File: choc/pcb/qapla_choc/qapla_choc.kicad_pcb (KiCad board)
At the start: 2 copper layers, 154.4 x 126.1 mm, 72 parts

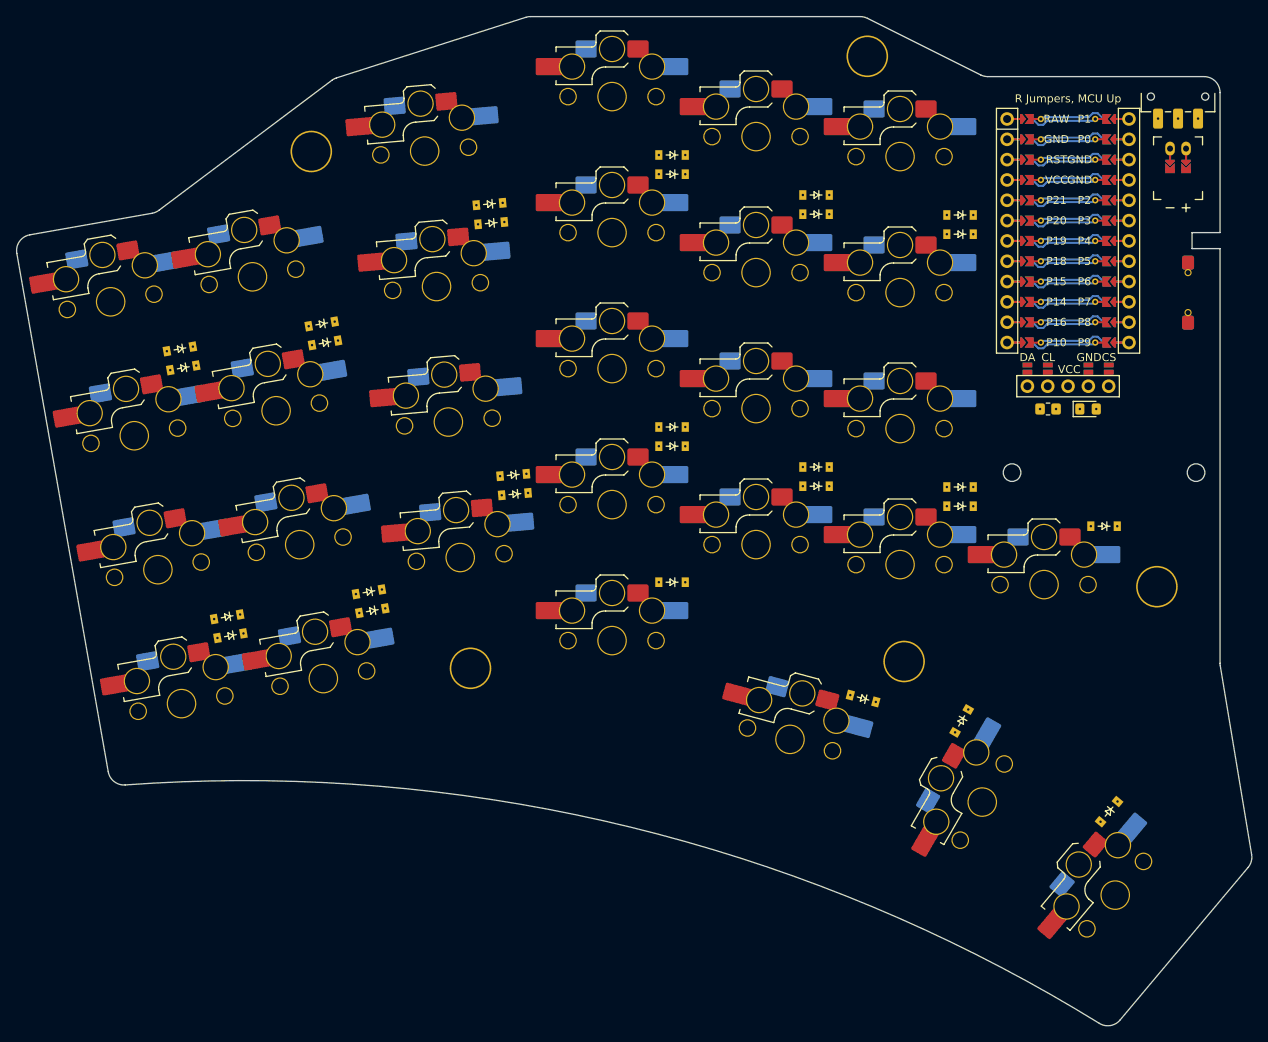
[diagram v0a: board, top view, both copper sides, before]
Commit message: MX Keyboard has a batleth
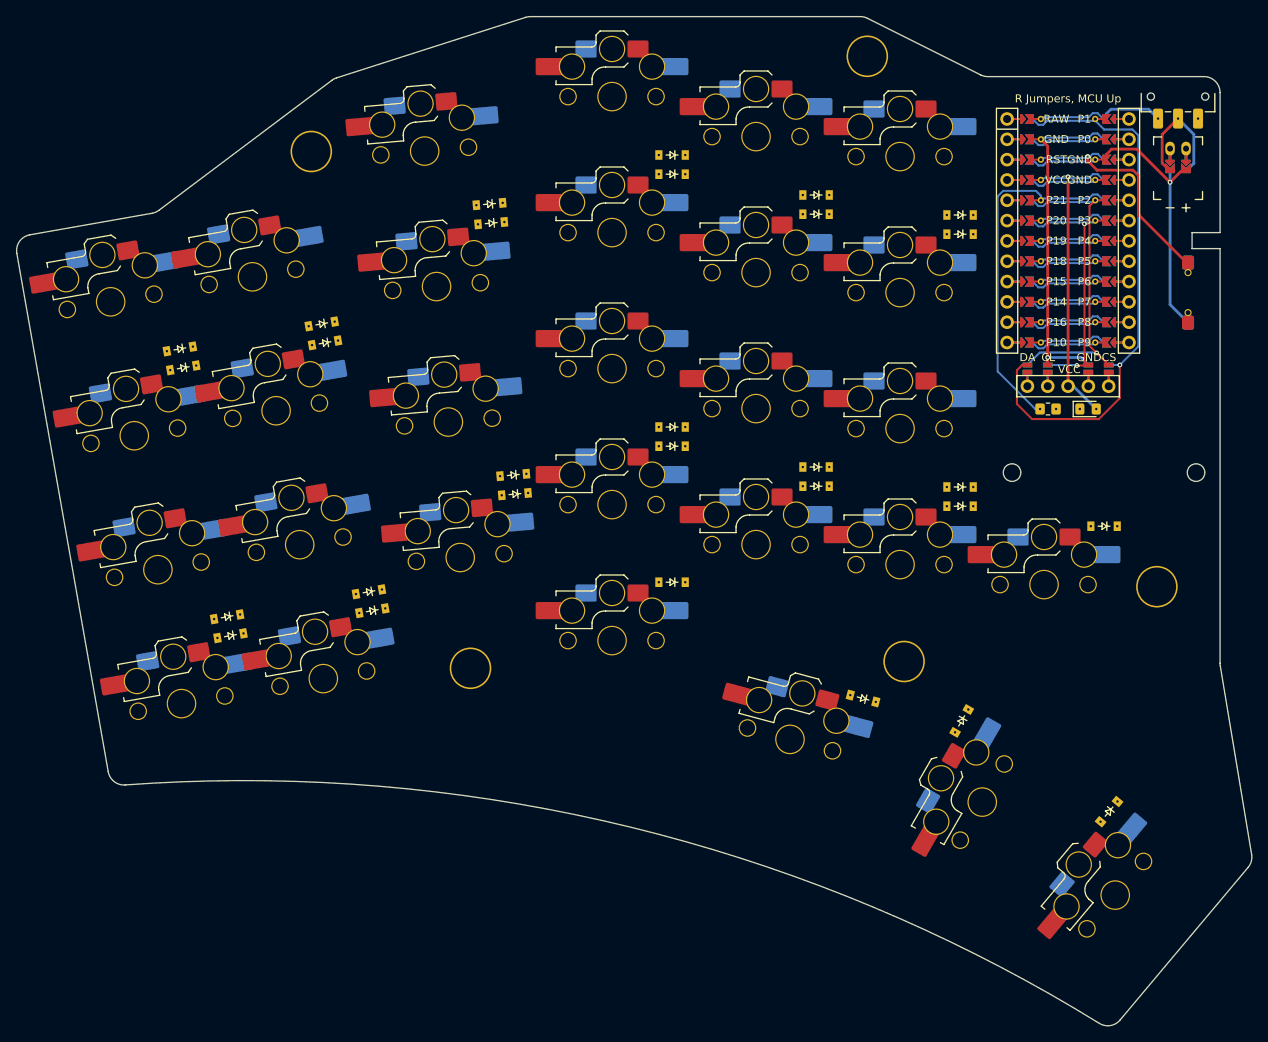
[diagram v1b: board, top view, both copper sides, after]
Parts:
- removed the _3 at (232.4, 76.8) (x2)
- added _3: , R_0805_2012Metric_Pad1.20x1.40mm_HandSolder, F.Cu at (232.4, 76.8)
- added _3: , D_0805_2012Metric_Pad1.15x1.40mm_HandSolder, F.Cu at (232.4, 76.8)
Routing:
- net (no net): track 337.7 -> 0.00 mm
- net GND: track 0.00 -> 96.6 mm, vias 0 -> 2
- net P1: track 0.00 -> 71.9 mm, vias 0 -> 1
- net P21: track 0.00 -> 45.5 mm
- net P2: track 0.00 -> 41.0 mm, vias 0 -> 1
- net VCC: track 0.00 -> 40.9 mm, vias 0 -> 1
- net P3: track 0.00 -> 32.8 mm, vias 0 -> 2
- net RST: track 0.00 -> 31.1 mm, vias 0 -> 1
- net RAW: track 0.00 -> 17.7 mm
- net BAT_P: track 0.00 -> 15.6 mm
- net P10: track 0.00 -> 9.84 mm
- net P20: track 0.00 -> 9.84 mm
- net P19: track 0.00 -> 9.84 mm
- net P18: track 0.00 -> 9.84 mm
- net P16: track 0.00 -> 9.84 mm
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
